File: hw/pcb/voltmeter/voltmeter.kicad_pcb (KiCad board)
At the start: 2 copper layers, 32 parts, among them J0 1935161, Q1 2N7002, Q2 2N7002, U1 SN74HC595DR, U2 TL062

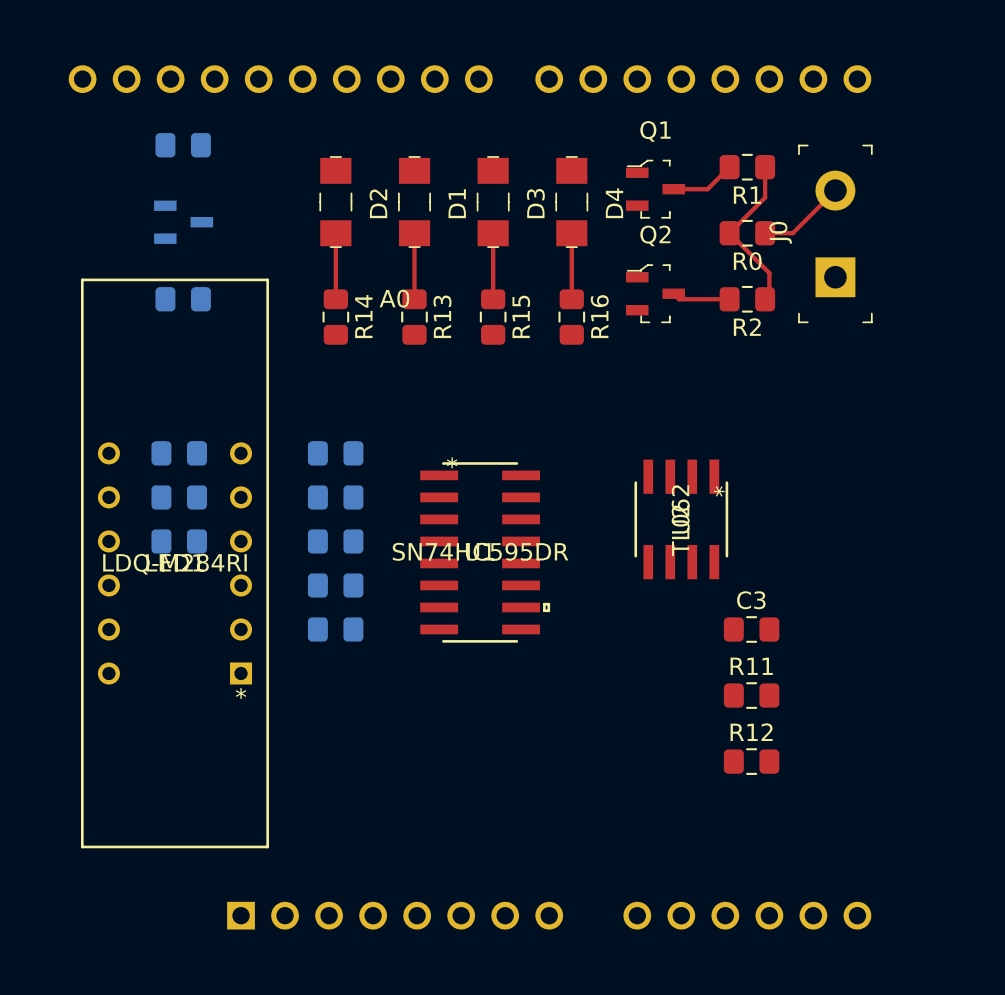
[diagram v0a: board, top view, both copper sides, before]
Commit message: Finished the layout!
Committing finalized layout.
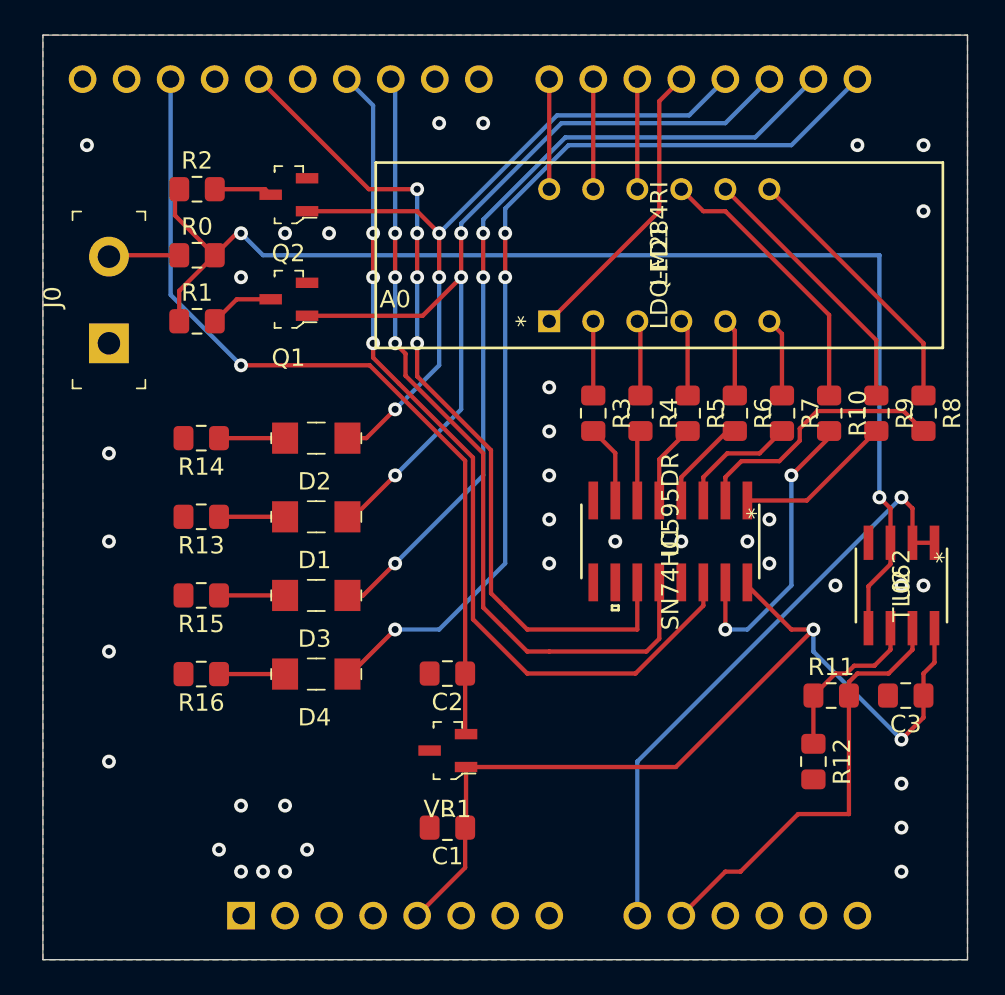
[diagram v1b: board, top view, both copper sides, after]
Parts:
- C1, C2, R10, R3, R4, R5, R6, R7, R8, R9, VR1: moved to F.Cu
- moved R8 43.0 mm to (165.1, 99.3), turned to 270 degrees
- moved J0 42.1 mm to (118.1, 95.2)
- moved R9 40.5 mm to (162.4, 99.3), turned to 270 degrees
- moved R10 38.2 mm to (159.7, 99.3), turned to 270 degrees
- moved C1 34.1 mm to (137.6, 123.2), turned to 180 degrees
- moved C2 34.1 mm to (137.6, 114.3), turned to 180 degrees
- moved VR1 34.1 mm to (137.7, 118.7), turned to 180 degrees
- moved R1 33.0 mm to (123.2, 94.0), turned to 0 degrees
- moved R2 32.4 mm to (123.2, 86.4), turned to 0 degrees
- moved R0 31.8 mm to (123.2, 90.2), turned to 0 degrees
- moved D4 31.0 mm to (130.1, 114.3), turned to 180 degrees
- moved R16 29.7 mm to (123.4, 114.3), turned to 180 degrees
- moved LED1 27.0 mm to (143.5, 94.0), turned to 90 degrees
- moved R7 25.8 mm to (156.9, 99.3), turned to 270 degrees
- moved D3 24.9 mm to (130.1, 109.8), turned to 180 degrees
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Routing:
- net /VoltageDivider: track 9.52 -> 71.2 mm, vias 0 -> 2
- net 1.2vLeg: track 0.00 -> 55.6 mm, vias 0 -> 3
- net VCC: track 0.00 -> 53.8 mm, vias 0 -> 2
- net Net-(A0-Pad26): track 0.00 -> 51.7 mm, vias 0 -> 3
- net 15vLeg: track 0.00 -> 50.9 mm, vias 0 -> 3
- net AREF_4.096v: track 0.00 -> 49.2 mm, vias 0 -> 1
- net Net-(A0-Pad28): track 0.00 -> 48.9 mm, vias 0 -> 4
- net 5vLeg: track 0.00 -> 47.9 mm, vias 0 -> 3
- net Net-(A0-Pad25): track 0.00 -> 47.5 mm, vias 0 -> 3
- net 30vLeg: track 0.00 -> 43.0 mm, vias 0 -> 3
- net ADC-Unity: track 0.00 -> 34.6 mm, vias 0 -> 1
- net ADC-Gain: track 0.00 -> 25.4 mm
- net Net-(R10-Pad2): track 0.00 -> 17.4 mm, vias 0 -> 2
- net Net-(A0-Pad19): track 0.00 -> 17.1 mm
- net Net-(LED1-Pad9): track 0.00 -> 16.2 mm
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- added copper zone on B.Cu, net GND
- added copper zone on F.Cu, net GND
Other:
- board outline added: 53.3 x 53.3 mm
- rule trace_min: 0.2 -> 0.1524
- rule via_min_size: 0.4 -> 0.1524
